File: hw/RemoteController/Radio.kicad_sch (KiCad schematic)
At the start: 89 parts, among them J4 BWSMA-KWE-Z3.5*4.2, U1 LM358, U10 H3-TCD-12-222X+, U16 H3-TCD-12-222X+, U17 AD8313xRM, U18 LM358, U3 SPF5043Z, U5 XA17-G4K, U6 MAX7044AKA, U8 AD8313xRM, U9 GVA-63, Y2 6.6128 MHz, Y3 10.7 MHz, Y4 13.56 MHz

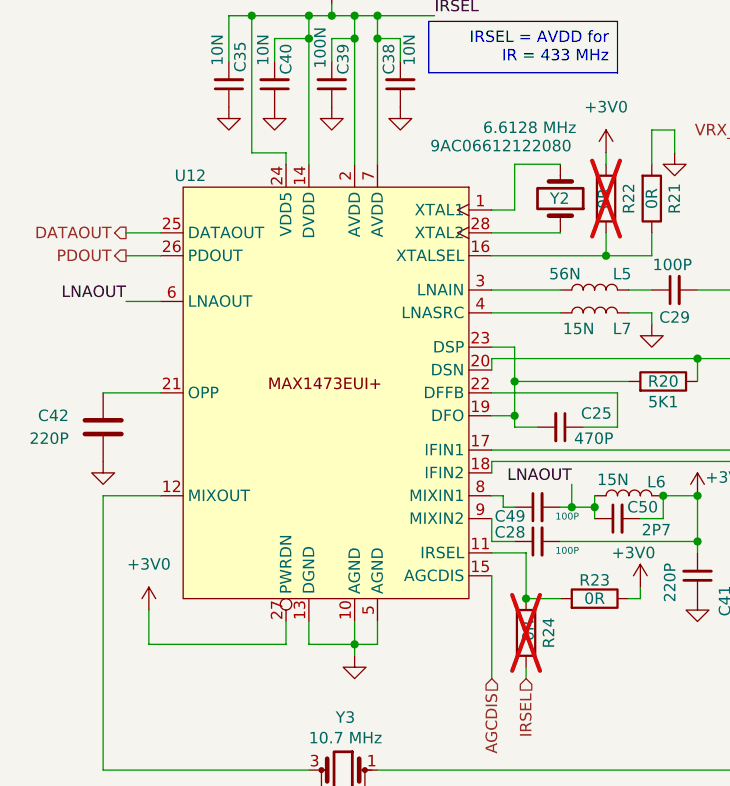
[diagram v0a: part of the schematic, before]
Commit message: remote_ctrl: re-start PCB
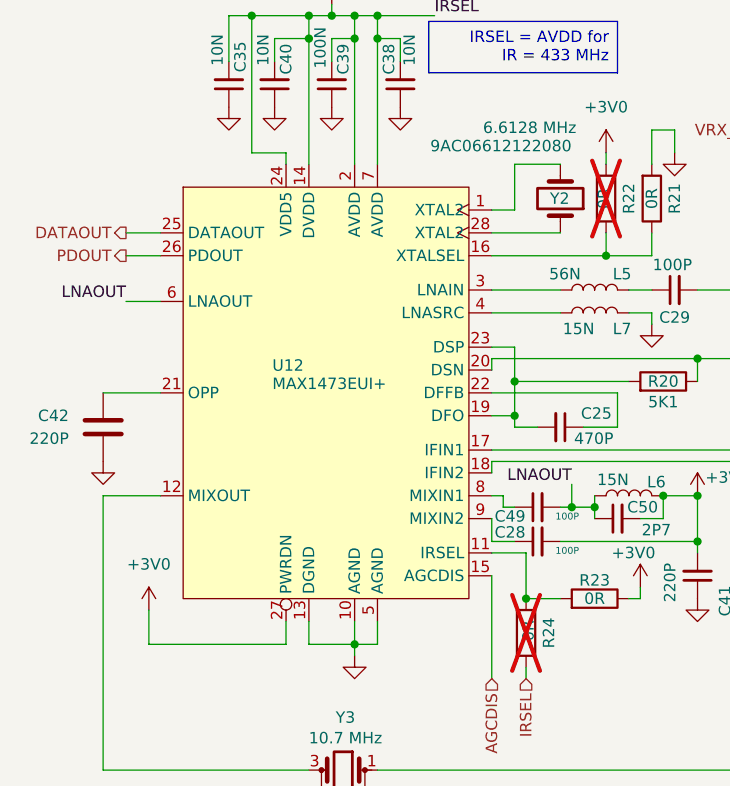
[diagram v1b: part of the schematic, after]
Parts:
- U12: value (none) -> MAX1473EUI+; footprint steew:MAX1473EUI+ -> Package_SO:TSSOP-28_4.4x9.7mm_P0.65mm
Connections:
- net at U16.4 (OUT): now also C29.2
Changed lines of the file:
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@@
-	)
-	(symbol
-		(lib_id "steew:MAX1473EUI+")
-		(at 64.77 121.92 0)
-		(mirror y)
-		(unit 1)
-		(body_style 1)
-		(exclude_from_sim no)
-		(in_bom yes)
-		(on_board yes)
-		(in_pos_files yes)
-		(dnp no)
-		(property "Reference" "U12"
-			(at 38.1 121.92 0)
-			(show_name no)
-			(do_not_autoplace no)
-			(effects
-				(font
-					(size 1.27 1.27)
-				)
-				(justify left)
-			)
-		)
-		(property "Value" ""
-			(at 44.8467 121.92 0)
-			(show_name no)
-			(do_not_autoplace no)
-			(effects
-				(font
-					(size 1.27 1.27)
-				)
-				(justify left)
-			)
-		)
-		(property "Footprint" "steew:MAX1473EUI+"
-			(at 64.77 121.92 0)
-			(hide yes)
-			(show_name no)
-			(do_not_autoplace no)
-			(effects
-				(font
-					(size 1.27 1.27)
-				)
-			)
-		)
-		(property "Datasheet" ""
-			(at 64.77 121.92 0)
-			(hide yes)
-			(show_name no)
-			(do_not_autoplace no)
-			(effects
-				(font
-					(size 1.27 1.27)
-				)
-			)
-		)
-		(property "Description" ""
-			(at 64.77 121.92 0)
-			(hide yes)
-			(show_name no)
-			(do_not_autoplace no)
-			(effects
-				(font
-					(size 1.27 1.27)
-				)
-			)
-		)
-		(pin "13"
-		)
-		(pin "25"
-		)
-		(pin "9"
-		)
-		(pin "15"
-		)
-		(pin "21"
-		)
-		(pin "26"
-		)
-		(pin "18"
-		)
-		(pin "19"
-		)
-		(pin "5"
-		)
-		(pin "10"
-		)
-		(pin "20"
-		)
-		(pin "14"
-		)
-		(pin "11"
-		)
-		(pin "12"
-		)
-		(pin "22"
-		)
-		(pin "23"
-		)
-		(pin "4"
-		)
-		(pin "3"
-		)
-		(pin "16"
-		)
-		(pin "28"
-		)
-		(pin "1"
-		)
-		(pin "7"
-		)
-		(pin "17"
-		)
-		(pin "24"
-		)
-		(pin "2"
-		)
-		(pin "8"
-		)
-		(pin "6"
-		)
-		(pin "27"
-		)
-		(instances
-			(project "RemoteController"
-				(path "/2496396e-da71-4b2e-9ac4-452e5130442d/d59aad70-30f5-48a2-8092-bdb11e43ed29"
-					(reference "U12")
-					(unit 1)
-				)
-			)
-		)
 	)
 	(symbol
@@
 					(unit 1)
 				)
+			)
+		)
+	)
+	(symbol
+		(lib_id "steew:MAX1473EUI+")
+		(at 52.07 123.19 0)
+		(unit 1)
+		(body_style 1)
+		(exclude_from_sim no)
+		(in_bom yes)
+		(on_board yes)
+		(in_pos_files yes)
+		(dnp no)
+		(property "Reference" "U12"
+			(at 45.466 143.002 0)
+			(show_name no)
+			(do_not_autoplace no)
+			(effects
+				(font
+					(size 1.27 1.27)
+				)
+				(justify left)
+			)
+		)
+		(property "Value" "MAX1473EUI+"
+			(at 45.466 145.034 0)
+			(show_name no)
+			(do_not_autoplace no)
+			(effects
+				(font
+					(size 1.27 1.27)
+				)
+				(justify left)
+			)
+		)
+		(property "Footprint" "Package_SO:TSSOP-28_4.4x9.7mm_P0.65mm"
+			(at 52.07 123.19 0)
+			(hide yes)
+			(show_name no)
+			(do_not_autoplace no)
+			(effects
+				(font
+					(size 1.27 1.27)
+				)
+			)
+		)
+		(property "Datasheet" "https://www.analog.com/media/en/technical-documentation/data-sheets/MAX1473.pdf"
+			(at 52.07 123.19 0)
+			(hide yes)
+			(show_name no)
+			(do_not_autoplace no)
+			(effects
+				(font
+					(size 1.27 1.27)
+				)
+			)
+		)
+		(property "Description" ""
+			(at 52.07 123.19 0)
+			(hide yes)
+			(show_name no)
+			(do_not_autoplace no)
+			(effects
+				(font
+					(size 1.27 1.27)
+				)
+			)
+		)
+		(pin "13"
+		)
+		(pin "25"
+		)
+		(pin "9"
+		)
+		(pin "15"
+		)
+		(pin "21"
+		)
+		(pin "26"
+		)
+		(pin "18"
+		)
+		(pin "19"
+		)
+		(pin "5"
+		)
+		(pin "10"
+		)
+		(pin "20"
+		)
+		(pin "14"
+		)
+		(pin "11"
+		)
+		(pin "12"
+		)
+		(pin "22"
+		)
+		(pin "23"
+		)
+		(pin "4"
+		)
+		(pin "3"
+		)
+		(pin "16"
+		)
+		(pin "28"
+		)
+		(pin "1"
+		)
+		(pin "7"
+		)
+		(pin "17"
+		)
+		(pin "24"
+		)
+		(pin "2"
+		)
+		(pin "8"
+		)
+		(pin "6"
+		)
+		(pin "27"
+		)
+		(instances
+			(project "RemoteController"
+				(path "/2496396e-da71-4b2e-9ac4-452e5130442d/d59aad70-30f5-48a2-8092-bdb11e43ed29"
+					(reference "U12")
+					(unit 1)
+				)
